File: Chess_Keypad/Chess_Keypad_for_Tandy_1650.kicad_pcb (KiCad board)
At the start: 2 copper layers, 150 x 73 mm, 113 parts, among them J1 Conn_02x09_Counter_Clockwise, J2 Conn_01x08, Q1 KSA992, Q2 KSA992, SW1 A8, SW10 B7, SW11 C7, SW12 D7, SW13 E7, SW14 F7, SW15 G7, SW16 H7, SW17 A6, SW18 B6, SW19 C6, SW2 B8, SW20 D6, SW21 E6, SW22 F6, SW23 G6, SW24 H6, SW25 A5, SW26 B5, SW27 C5, SW28 D5, SW29 E5, SW3 C8, SW30 F5, SW31 G5, SW32 H5, SW33 A4, SW34 B4, SW35 C4, SW36 D4, SW37 E4, SW38 F4, SW39 G4, SW4 D8, SW40 H4, SW41 A3, SW42 B3, SW43 C3, SW44 D3, SW45 E3, SW46 F3, SW47 G3, SW48 H3, SW49 A2, SW5 E8, SW50 B2, SW51 C2, SW52 D2, SW53 E2, SW54 F2, SW55 G2, SW56 H2, SW57 A1, SW58 B1, SW59 C1, SW6 F8, SW60 D1, SW61 E1, SW62 F1, SW63 G1, SW64 H1, SW65 COLOUR, SW66 NEW GAME, SW67 2ndF, SW68 KING, SW69 ROOK, SW7 G8, SW70 BISHOP, SW71 TAKE BACK, SW72 LEVEL, SW73 PLAY, SW74 KNIGHT, SW75 PAWN, SW76 QUEEN, SW8 H8, SW9 A7

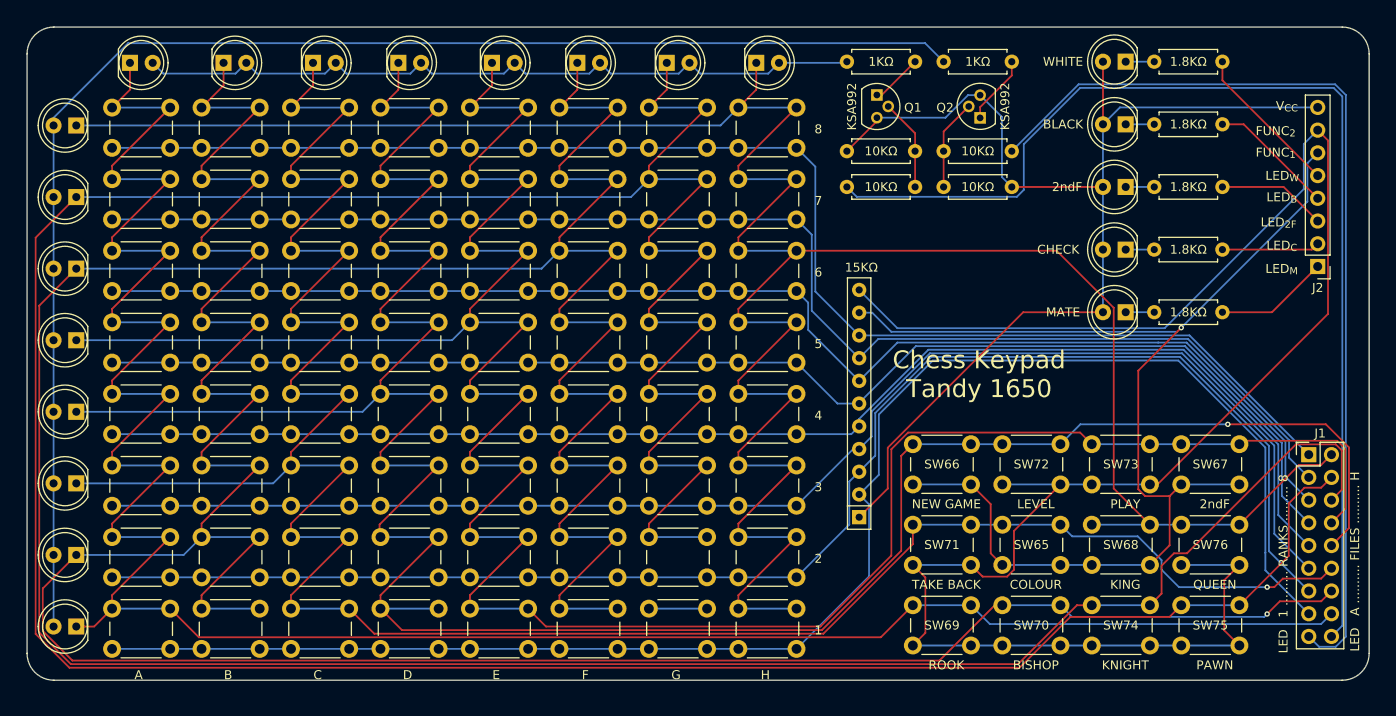
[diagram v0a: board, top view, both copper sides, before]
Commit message: Finalised initial design
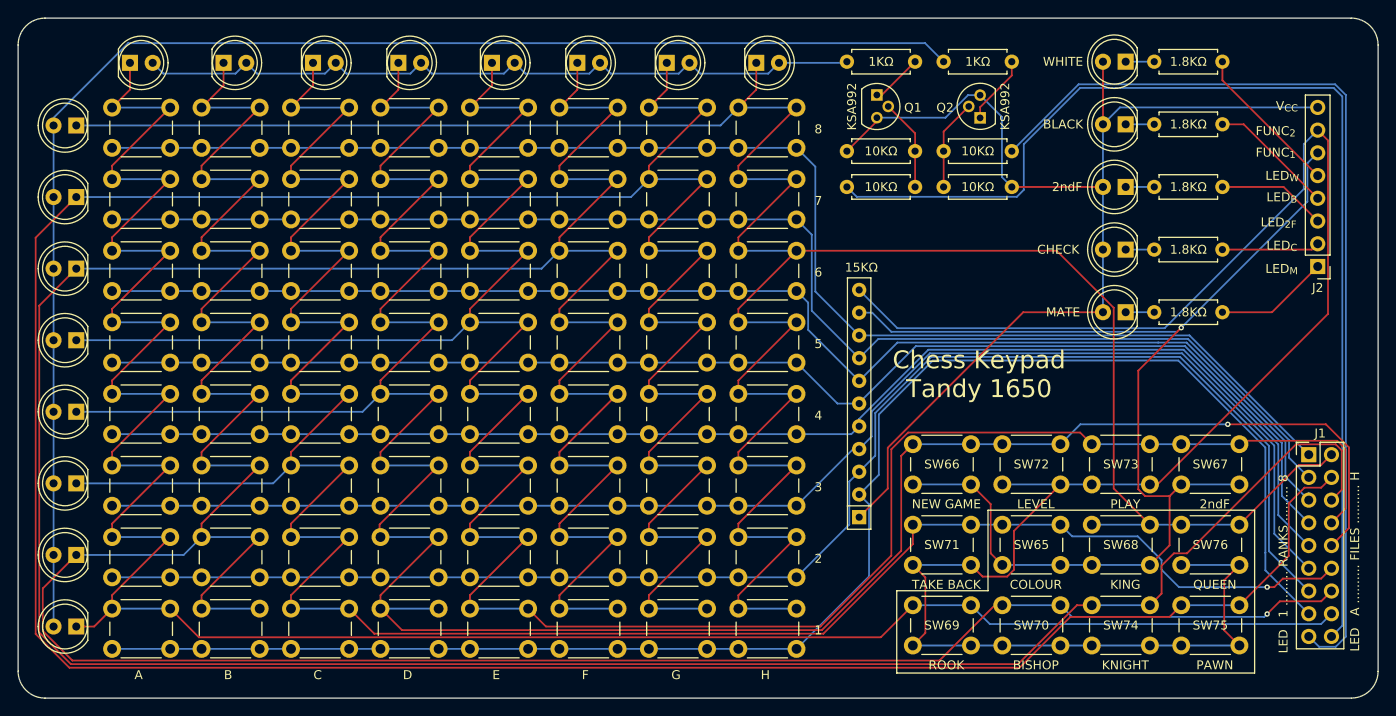
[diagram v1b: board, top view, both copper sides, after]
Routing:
- net /FILE_{G}: track 396.2 -> 406.9 mm
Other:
- board size 150 x 73 mm -> 152 x 76 mm
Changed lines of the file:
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@@
 	)
 	(gr_line
-		(start 198.25 50.25)
-		(end 198.25 117.25)
+		(start 185.45 119.45)
+		(end 185.45 101.25)
+		(stroke
+			(width 0.1)
+			(type default)
+		)
+		(layer "F.SilkS")
+	)
+	(gr_line
+		(start 185.45 101.25)
+		(end 155.65 101.25)
+		(stroke
+			(width 0.1)
+			(type default)
+		)
+		(layer "F.SilkS")
+	)
+	(gr_line
+		(start 155.65 101.25)
+		(end 155.65 110.25)
+		(stroke
+			(width 0.1)
+			(type default)
+		)
+		(layer "F.SilkS")
+	)
+	(gr_line
+		(start 145.45 119.45)
+		(end 185.45 119.45)
+		(stroke
+			(width 0.1)
+			(type default)
+		)
+		(layer "F.SilkS")
+	)
+	(gr_line
+		(start 155.65 110.25)
+		(end 145.45 110.25)
+		(stroke
+			(width 0.1)
+			(type default)
+		)
+		(layer "F.SilkS")
+	)
+	(gr_line
+		(start 145.45 110.25)
+		(end 145.45 119.45)
+		(stroke
+			(width 0.1)
+			(type default)
+		)
+		(layer "F.SilkS")
+	)
+	(gr_line
+		(start 47.25 119.25)
+		(end 47.25 49.25)
 		(stroke
 			(width 0.05)
@@
 	)
 	(gr_line
-		(start 51.25 47.25)
-		(end 195.25 47.25)
+		(start 199.25 49.25)
+		(end 199.25 119.25)
 		(stroke
 			(width 0.05)
@@
 	)
 	(gr_arc
-		(start 198.25 117.25)
-		(mid 197.37132 119.37132)
-		(end 195.25 120.25)
+		(start 50.25 122.25)
+		(mid 48.12868 121.37132)
+		(end 47.25 119.25)
 		(stroke
 			(width 0.05)
@@
 	)
 	(gr_arc
-		(start 195.25 47.25)
-		(mid 197.37132 48.12868)
-		(end 198.25 50.25)
+		(start 47.25 49.25)
+		(mid 48.12868 47.12868)
+		(end 50.25 46.25)
 		(stroke
 			(width 0.05)
@@
 		(layer "Edge.Cuts")
 	)
-	(gr_arc
-		(start 48.25 50.25)
-		(mid 49.12868 48.12868)
-		(end 51.25 47.25)
+	(gr_line
+		(start 196.25 122.25)
+		(end 50.25 122.25)
 		(stroke
 			(width 0.05)
@@
 		(layer "Edge.Cuts")
 	)
-	(gr_line
-		(start 48.25 117.25)
-		(end 48.25 50.25)
+	(gr_arc
+		(start 199.25 119.25)
+		(mid 198.37132 121.37132)
+		(end 196.25 122.25)
 		(stroke
 			(width 0.05)
@@
 	)
 	(gr_arc
-		(start 51.25 120.25)
-		(mid 49.12868 119.37132)
-		(end 48.25 117.25)
+		(start 196.25 46.25)
+		(mid 198.37132 47.12868)
+		(end 199.25 49.25)
 		(stroke
 			(width 0.05)
@@
 	)
 	(gr_line
-		(start 195.25 120.25)
-		(end 51.25 120.25)
+		(start 50.25 46.25)
+		(end 196.25 46.25)
 		(stroke
 			(width 0.05)
@@
 	)
 	(segment
+		(start 124.25 104.25)
+		(end 117.75 110.75)
+		(width 0.2)
+		(layer "F.Cu")
+		(net 9)
+	)
+	(segment
 		(start 117.75 94.75)
 		(end 117.75 96.25)
@@
 		(width 0.2)
 		(layer "F.Cu")
+		(net 9)
+	)
+	(segment
+		(start 117.75 110.75)
+		(end 117.75 112.25)
+		(width 0.2)
+		(layer "F.Cu")
